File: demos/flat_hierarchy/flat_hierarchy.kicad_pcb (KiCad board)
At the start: 2 copper layers, 160 x 99.1 mm, 64 parts, among them J1 DB9-FEMAL, P1 CONN_2, P2 SUPP28, P3 SUPP40, Q1 BC237, Q2 BC307, Q3 BC307, U1 24Cxx, U2 74HC125, U3 7805, U4 LT1373, U5 PIC_18_PINS, U6 PIC_8_PINS

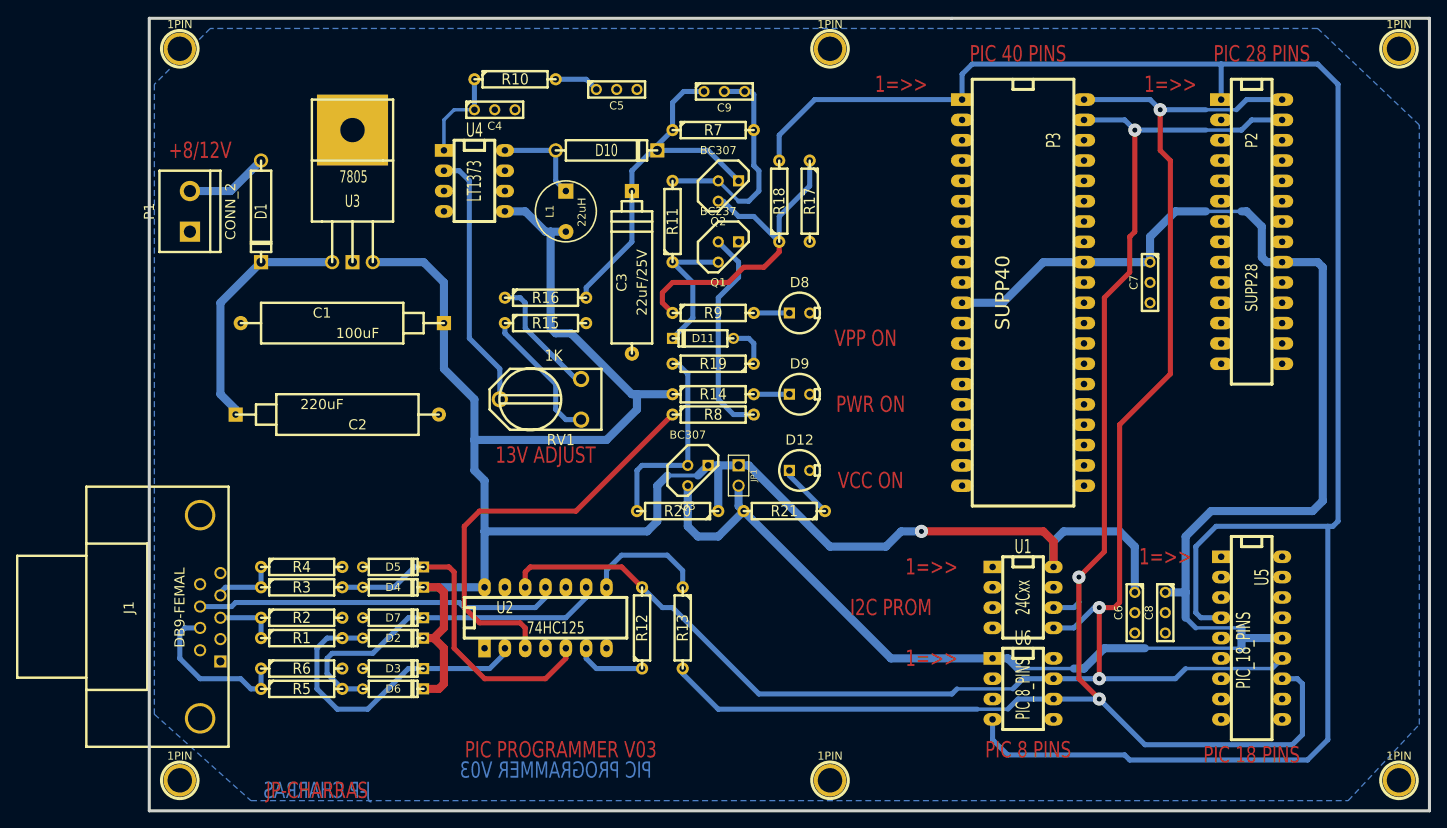
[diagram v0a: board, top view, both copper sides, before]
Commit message: New upstream version 5.0.0~rc1+dfsg1
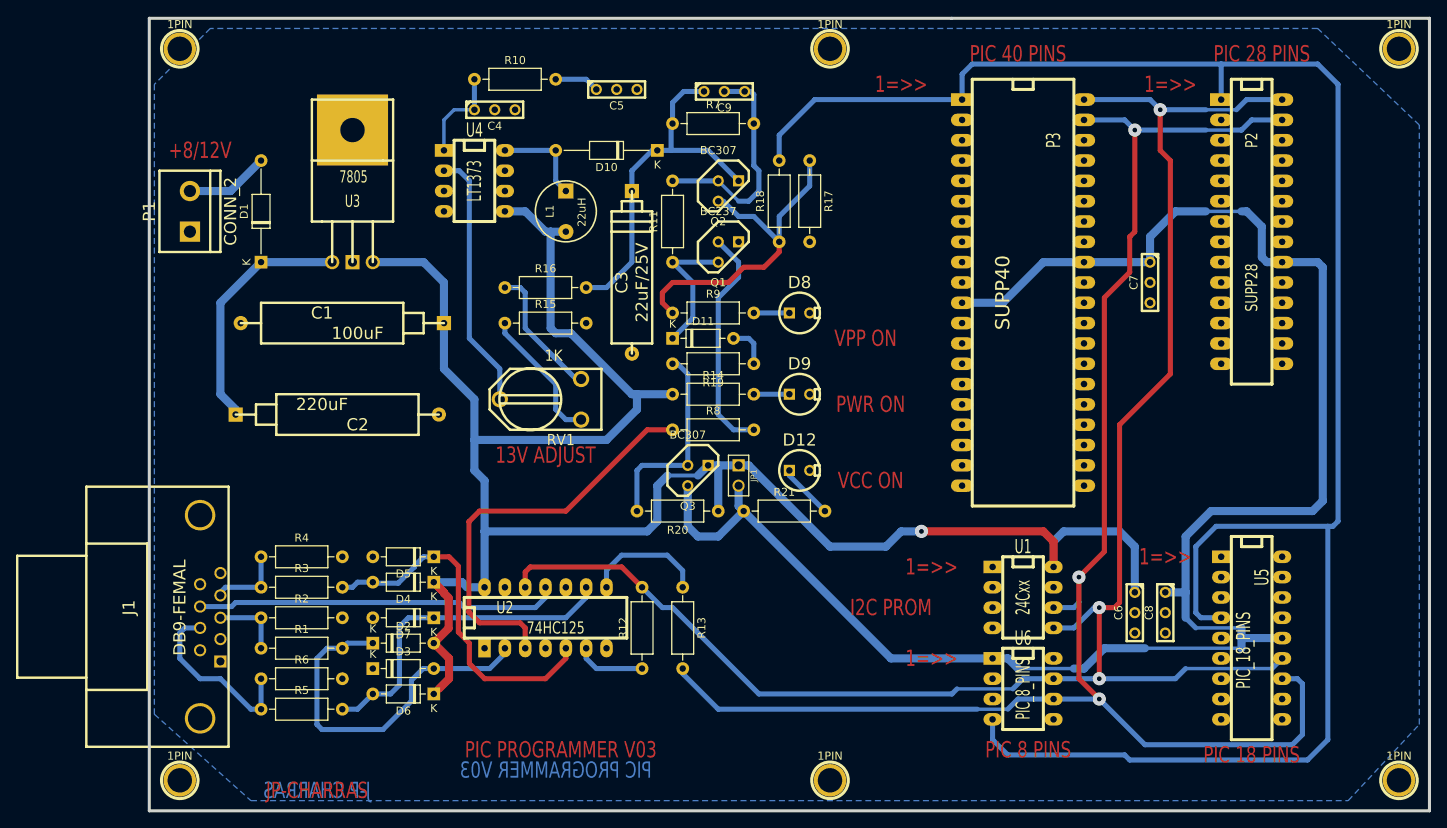
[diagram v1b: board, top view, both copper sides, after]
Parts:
- D1, D10: footprint discret:D5 -> Diode_THT:D_DO-35_SOD27_P12.70mm_Horizontal
- D11, D2, D3, D4, D5, D6, D7: footprint discret:D3 -> Diode_THT:D_DO-35_SOD27_P7.62mm_Horizontal
- R1, R11, R12, R13, R14, R15, R16, R17, R18, R19, R2, R20, R21, R3, R4, R5, R6, R7, R8, R9: footprint discret:R4 -> Resistor_THT:R_Axial_DIN0207_L6.3mm_D2.5mm_P10.16mm_Horizontal
- R10: value 5,1K -> 5.1K; footprint discret:R4 -> Resistor_THT:R_Axial_DIN0207_L6.3mm_D2.5mm_P10.16mm_Horizontal
- moved D1 6.35 mm to (87.6, 71.1), turned to 90 degrees
- moved D10 6.35 mm to (137.2, 57.1), turned to 180 degrees
- moved R5 5.68 mm to (87.6, 127.0)
- moved R8 5.43 mm to (139.1, 92.1)
- moved D5 5.24 mm to (109.2, 108.0), turned to 180 degrees
- moved R1 5.24 mm to (87.6, 119.4)
- moved R16 5.24 mm to (118.1, 74.3)
- moved R4 5.24 mm to (87.6, 108.0)
- moved R6 5.24 mm to (87.6, 123.2)
- moved R7 5.14 mm to (139.1, 53.8)
- moved D4 5.12 mm to (109.2, 111.1), turned to 180 degrees
- moved D6 5.12 mm to (109.2, 125.1), turned to 180 degrees
- moved R14 5.08 mm to (139.1, 87.6)
- moved R20 5.08 mm to (144.8, 102.2)
- moved R9 5.08 mm to (139.1, 77.5)
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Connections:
- D1 pad 1: Net-(D1-Pad1) -> Net-(C2-Pad1)
- D1 pad 2: Net-(C2-Pad1) -> Net-(D1-Pad2)
- D10 pad 1: Net-(D10-Pad1) -> VPP
- D10 pad 2: VPP -> Net-(D10-Pad2)
- D4 pad 1: Net-(D4-Pad1) -> VCC
- D4 pad 2: VCC -> Net-(D4-Pad2)
- D5 pad 1: GND -> Net-(D4-Pad2)
- D5 pad 2: Net-(D4-Pad1) -> GND
- D6 pad 1: Net-(D6-Pad1) -> VCC
- D6 pad 2: VCC -> Net-(D6-Pad2)
- D7 pad 1: GND -> Net-(D6-Pad2)
- D7 pad 2: Net-(D6-Pad1) -> GND
- J1 pad 1: (no net) -> Net-(J1-Pad1)
- J1 pad 2: (no net) -> Net-(J1-Pad2)
- J1 pad 6: (no net) -> Net-(J1-Pad6)
- J1 pad 9: (no net) -> Net-(J1-Pad9)
- L1 pad 1: Net-(D10-Pad1) -> Net-(D10-Pad2)
- P1 pad 2: Net-(D1-Pad1) -> Net-(D1-Pad2)
- P2 pad 10: (no net) -> Net-(P2-Pad10)
- P2 pad 11: (no net) -> Net-(P2-Pad11)
- P2 pad 12: (no net) -> Net-(P2-Pad12)
- P2 pad 13: (no net) -> Net-(P2-Pad13)
- P2 pad 14: (no net) -> Net-(P2-Pad14)
- P2 pad 15: (no net) -> Net-(P2-Pad15)
- P2 pad 16: (no net) -> Net-(P2-Pad16)
- P2 pad 17: (no net) -> Net-(P2-Pad17)
- P2 pad 18: (no net) -> Net-(P2-Pad18)
- P2 pad 2: (no net) -> Net-(P2-Pad2)
- P2 pad 21: (no net) -> Net-(P2-Pad21)
- P2 pad 22: (no net) -> Net-(P2-Pad22)
- P2 pad 23: (no net) -> Net-(P2-Pad23)
- P2 pad 24: (no net) -> Net-(P2-Pad24)
- P2 pad 25: (no net) -> Net-(P2-Pad25)
- P2 pad 26: (no net) -> Net-(P2-Pad26)
- P2 pad 3: (no net) -> Net-(P2-Pad3)
- P2 pad 4: (no net) -> Net-(P2-Pad4)
- P2 pad 5: (no net) -> Net-(P2-Pad5)
- P2 pad 6: (no net) -> Net-(P2-Pad6)
- P2 pad 7: (no net) -> Net-(P2-Pad7)
- P2 pad 9: (no net) -> Net-(P2-Pad9)
- P3 pad 10: (no net) -> Net-(P3-Pad10)
- P3 pad 13: (no net) -> Net-(P3-Pad13)
- P3 pad 14: (no net) -> Net-(P3-Pad14)
- P3 pad 15: (no net) -> Net-(P3-Pad15)
- P3 pad 16: (no net) -> Net-(P3-Pad16)
- P3 pad 17: (no net) -> Net-(P3-Pad17)
- P3 pad 18: (no net) -> Net-(P3-Pad18)
- P3 pad 19: (no net) -> Net-(P3-Pad19)
- P3 pad 2: (no net) -> Net-(P3-Pad2)
- P3 pad 20: (no net) -> Net-(P3-Pad20)
- P3 pad 21: (no net) -> Net-(P3-Pad21)
- P3 pad 22: (no net) -> Net-(P3-Pad22)
- P3 pad 23: (no net) -> Net-(P3-Pad23)
- P3 pad 24: (no net) -> Net-(P3-Pad24)
- P3 pad 25: (no net) -> Net-(P3-Pad25)
- P3 pad 26: (no net) -> Net-(P3-Pad26)
- P3 pad 27: (no net) -> Net-(P3-Pad27)
- P3 pad 28: (no net) -> Net-(P3-Pad28)
- P3 pad 29: (no net) -> Net-(P3-Pad29)
- P3 pad 3: (no net) -> Net-(P3-Pad3)
- P3 pad 30: (no net) -> Net-(P3-Pad30)
- P3 pad 33: (no net) -> Net-(P3-Pad33)
- P3 pad 34: (no net) -> Net-(P3-Pad34)
- P3 pad 35: (no net) -> Net-(P3-Pad35)
- P3 pad 36: (no net) -> Net-(P3-Pad36)
- P3 pad 37: (no net) -> Net-(P3-Pad37)
- P3 pad 38: (no net) -> Net-(P3-Pad38)
- P3 pad 4: (no net) -> Net-(P3-Pad4)
- P3 pad 5: (no net) -> Net-(P3-Pad5)
- P3 pad 6: (no net) -> Net-(P3-Pad6)
- P3 pad 7: (no net) -> Net-(P3-Pad7)
- P3 pad 9: (no net) -> Net-(P3-Pad9)
- Q1 pad 3: Net-(D11-Pad2) -> Net-(D11-Pad1)
- R11 pad 1: Net-(D11-Pad2) -> Net-(D11-Pad1)
- R19 pad 1: Net-(D11-Pad1) -> Net-(D11-Pad2)
- R21 pad 1: Net-(D12-Pad1) -> VCC_PIC
- R21 pad 2: VCC_PIC -> Net-(D12-Pad1)
- R3 pad 2: Net-(D4-Pad1) -> Net-(D4-Pad2)
- R5 pad 2: Net-(D6-Pad1) -> Net-(D6-Pad2)
- U1 pad 7: (no net) -> Net-(U1-Pad7)
- U2 pad 5: Net-(D4-Pad1) -> Net-(D4-Pad2)
- U2 pad 9: Net-(D6-Pad1) -> Net-(D6-Pad2)
- U4 pad 3: (no net) -> Net-(U4-Pad3)
- U4 pad 4: (no net) -> Net-(U4-Pad4)
- U4 pad 8: Net-(D10-Pad1) -> Net-(D10-Pad2)
- U5 pad 1: (no net) -> Net-(U5-Pad1)
- U5 pad 10: (no net) -> Net-(U5-Pad10)
- U5 pad 11: (no net) -> Net-(U5-Pad11)
- U5 pad 15: (no net) -> Net-(U5-Pad15)
- U5 pad 16: (no net) -> Net-(U5-Pad16)
- U5 pad 17: (no net) -> Net-(U5-Pad17)
- U5 pad 18: (no net) -> Net-(U5-Pad18)
- U5 pad 2: (no net) -> Net-(U5-Pad2)
- U5 pad 3: (no net) -> Net-(U5-Pad3)
- U5 pad 6: (no net) -> Net-(U5-Pad6)
- U5 pad 7: (no net) -> Net-(U5-Pad7)
- U5 pad 8: (no net) -> Net-(U5-Pad8)
- U5 pad 9: (no net) -> Net-(U5-Pad9)
- U6 pad 2: (no net) -> Net-(U6-Pad2)
- U6 pad 3: (no net) -> Net-(U6-Pad3)
- U6 pad 5: (no net) -> Net-(U6-Pad5)
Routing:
- net Net-(D4-Pad2): track 0.00 -> 44.7 mm
- net Net-(D6-Pad1): track 44.0 -> 0.00 mm
- net Net-(D4-Pad1): track 42.7 -> 0.00 mm
- net Net-(D6-Pad2): track 0.00 -> 41.8 mm
- net Net-(D11-Pad2): track 17.3 -> 5.34 mm
- net Net-(D11-Pad1): track 5.34 -> 17.3 mm
- net Net-(D10-Pad2): track 0.00 -> 12.0 mm
- net Net-(D10-Pad1): track 12.0 -> 0.00 mm
- net Net-(D1-Pad2): track 0.00 -> 10.5 mm
- net Net-(D1-Pad1): track 10.5 -> 0.00 mm
- net Net-(D2-Pad1): track 39.4 -> 45.9 mm
- net VCC: track 252.2 -> 249.0 mm
- net /pic_programmer/PC-CLOCK-OUT: track 20.3 -> 22.6 mm
- net Net-(Q1-Pad2): track 27.0 -> 28.9 mm
- net Net-(R8-Pad1): track 53.2 -> 51.9 mm
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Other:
- net class Default: trace_width 0.254 -> 0.4; via_dia 0.889 -> 0.9; via_drill 0.635 -> 0.6
- rule trace_min: 0.254 -> 0.2
- rule via_min_size: 0.889 -> 0.8
